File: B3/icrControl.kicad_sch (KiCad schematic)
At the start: 12 parts, among them U329 74HC00, U330 74HC74, U331 74HC74, U332 74HC74, U333 74HC74, U334 74HC74, U335 74HCT04, U336 74HC244, U337 74HC08, U338 74HC32, U339 74HC08, U341 74HC157

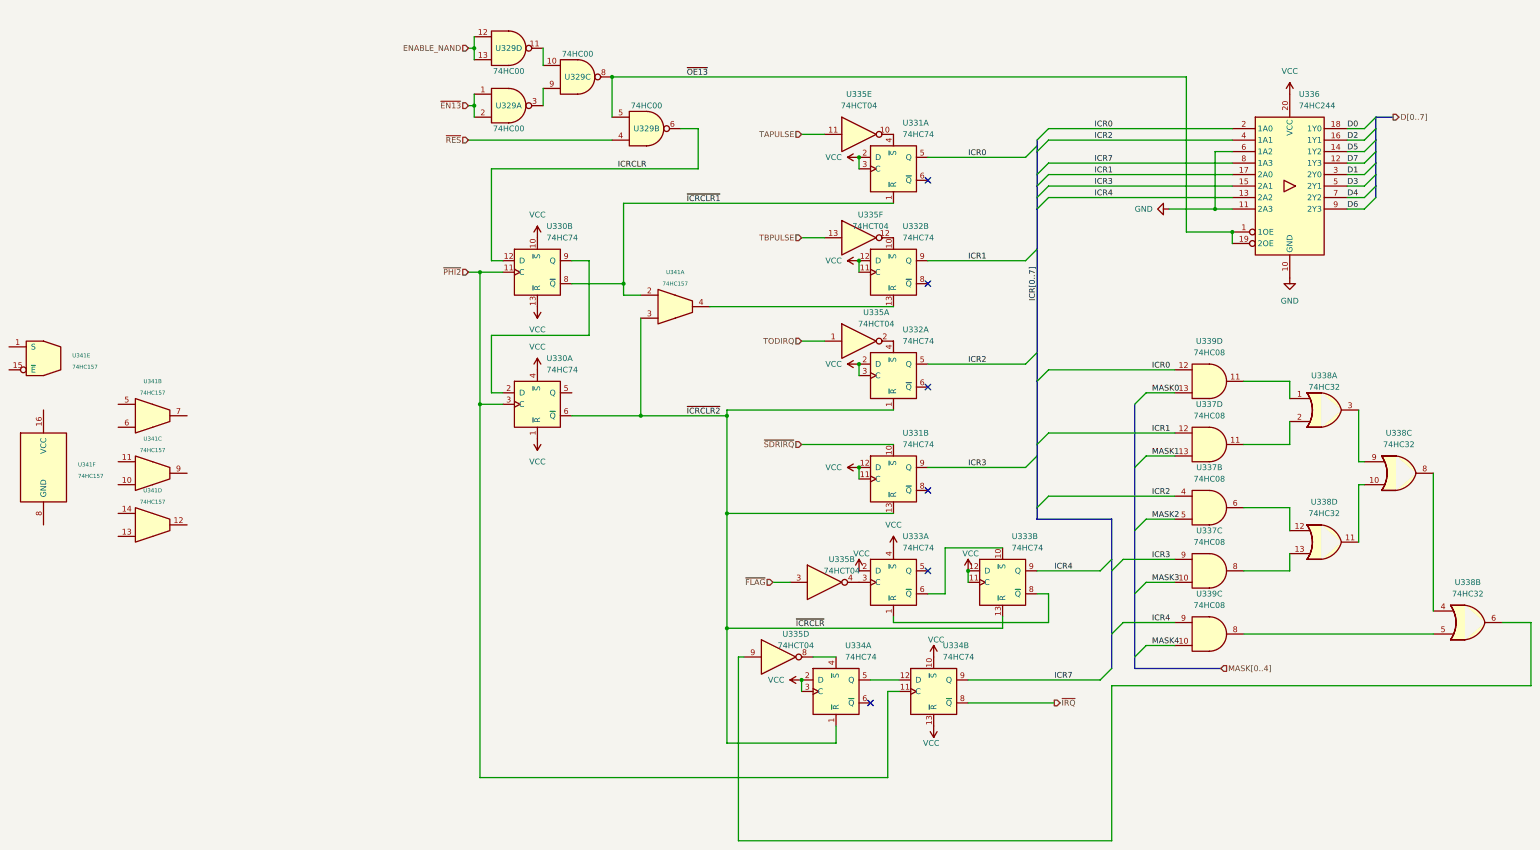
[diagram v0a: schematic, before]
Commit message: Ready for v0.2.2
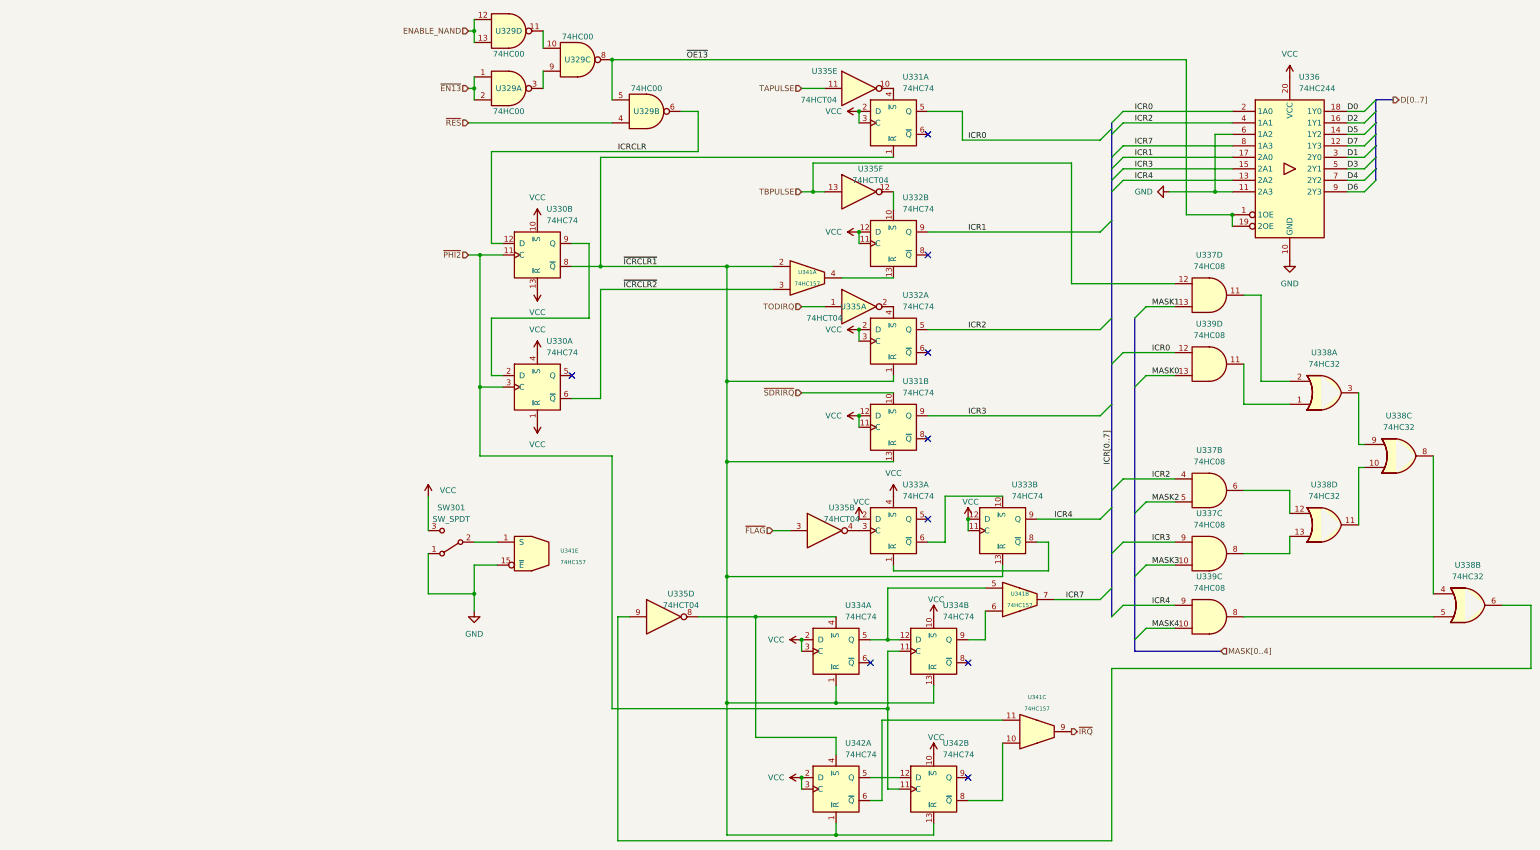
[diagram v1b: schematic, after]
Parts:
- removed unit 4 of U341
- removed unit 6 of U341
- added SW301: SW_SPDT, Button_Switch_SMD:SW_SPDT_PCM12, symbol Switch:SW_SPDT
- added U342: 74HC74, Package_SO:SO-14_3.9x8.65mm_P1.27mm, symbol 74xx:74HC74
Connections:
- net GND: now also U341.15 (~{E}), SW301.1 (A)
- net ICR1: no longer U337.12
- net ICR7: now also U341.7; no longer U334.9 (Q)
- net TBPULSE: now also U337.12
- net VCC: now also SW301.3 (C), U342.10 (~{S}), U342.2 (D), U342.3 (C); no longer U334.13 (~{R})
- net ~{ICRCLR1}: now also U331.13 (~{R}), U332.1 (~{R}), U333.13 (~{R}), U334.1 (~{R}), U334.13 (~{R}), U342.1 (~{R}), U342.13 (~{R})
- net ~{ICRCLR2}: no longer U331.13 (~{R}), U332.1 (~{R}), U333.13 (~{R}), U334.1 (~{R})
- net ~{IRQ}: now also U341.9; no longer U334.8 (~{Q})
- net ~{PHI2}: now also U342.11 (C)
- net at U341.5: now also U334.12 (D), U334.5 (Q)
- net at U341.6: now also U334.9 (Q)
- net at U334.4 (~{S}), U335.8: now also U342.4 (~{S})
- net at U341.1 (S): now also SW301.2 (B)
- net at U341.10: now also U342.8 (~{Q})
- net at U341.11: now also U342.6 (~{Q})
- new net: U342.12 (D), U342.5 (Q)
- no-connect marks 6 -> 9
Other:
- moved on the sheet: U329A, U329B, U329C, U329D, U330A, U330B, U331A, U331B, U332A, U332B, U333A, U333B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
